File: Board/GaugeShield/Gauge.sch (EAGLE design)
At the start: 29 parts

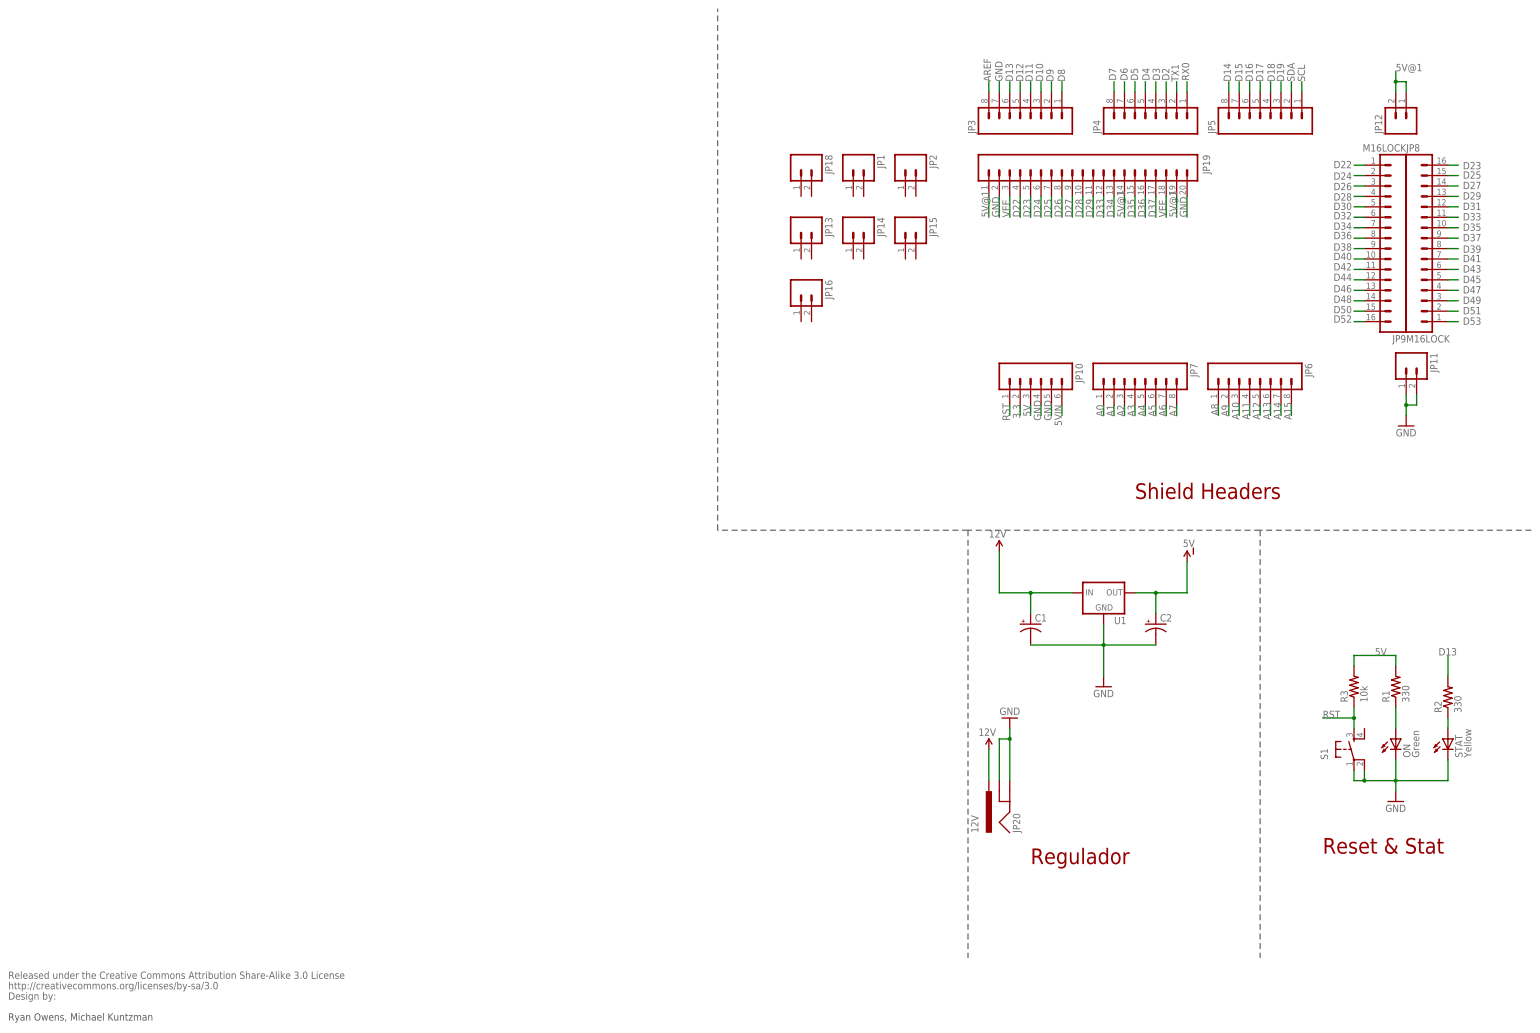
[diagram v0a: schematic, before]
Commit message: empece a diagramar la parte del board y a tracear las rutas
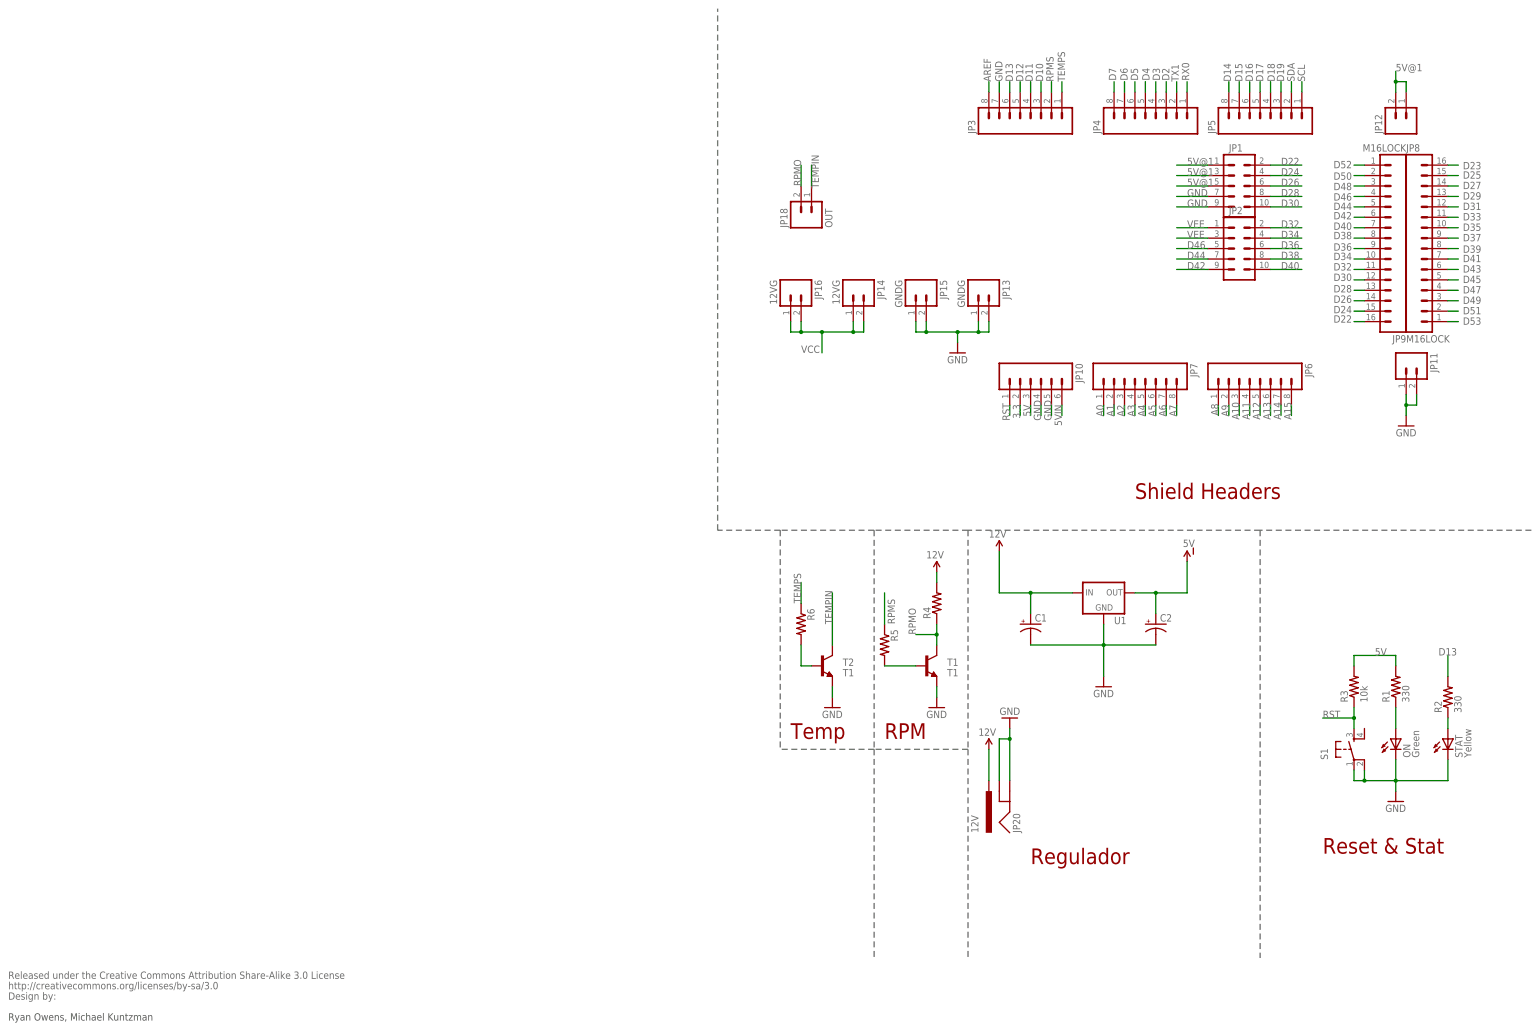
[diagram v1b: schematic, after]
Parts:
- removed JP19: (no value), SparkFun-Connectors:M20
- added R4, R5, R6: (no value), SparkFun-Passives:RESISTORPTH-1/2W
- added T1, T2: T1, SparkFun-DiscreteSemi:TRANSISTOR_NPN_2PTH
- JP1, JP2: device SparkFun-Connectors:M02POLAR -> SparkFun-Connectors:M05X2PTH
- JP13, JP15: value (none) -> GNDG
- JP14, JP16: value (none) -> 12VG
- JP18: value (none) -> OUT
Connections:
- removed net D8: JP3.1
- removed net D9: JP3.2
- new net N$1: R5.2, T1.B
- new net N$2: R6.2, T2.B
- new net RPMO: JP18.2, R4.1, T1.C
- new net RPMS: JP3.2, R5.1
- new net TEMPIN: JP18.1, T2.C
- new net TEMPS: JP3.1, R6.1
- new net VCC: C1.+, JP14.1, JP14.2, JP16.1, JP16.2, JP20.PWR, U1.IN
- net 5V@1: now also JP1.1, JP1.3, JP1.5; no longer JP19.1, JP19.14, JP19.19
- net D22: now also JP1.2, JP9.16; no longer JP19.4, JP9.1
- net D23: no longer JP19.5
- net D24: now also JP1.4, JP9.15; no longer JP19.6, JP9.2
- net D25: no longer JP19.7
- net D26: now also JP1.6, JP9.14; no longer JP19.8, JP9.3
- net D27: no longer JP19.9
- net D28: now also JP1.8, JP9.13; no longer JP19.10, JP9.4
- net D29: no longer JP19.11
- net D30: now also JP1.10, JP9.12; no longer JP9.5
- net D32: now also JP2.2, JP9.11; no longer JP9.6
- net D33: no longer JP19.12
- net D34: now also JP2.4, JP9.10; no longer JP19.13, JP9.7
- net D35: no longer JP19.15
- net D36: now also JP2.6, JP9.9; no longer JP19.16, JP9.8
- net D37: no longer JP19.17
- net D38: now also JP2.8, JP9.8; no longer JP9.9
- net D40: now also JP2.10, JP9.7; no longer JP9.10
- net D42: now also JP2.9, JP9.6; no longer JP9.11
- net D44: now also JP2.7, JP9.5; no longer JP9.12
- net D46: now also JP2.5, JP9.4; no longer JP9.13
- net D48: now also JP9.3; no longer JP9.14
- net D50: now also JP9.2; no longer JP9.15
- net D52: now also JP9.1; no longer JP9.16
- net GND: now also JP1.7, JP1.9, JP13.1, JP13.2, JP15.1, JP15.2, T1.E, T2.E; no longer JP19.2, JP19.20
- net VEE: now also JP2.1, JP2.3; no longer JP19.18, JP19.3
- net VNEG: now also R4.2; no longer C1.+, JP20.PWR, U1.IN
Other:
- note added: "RPM"
- note added: "Temp"
- moved on the sheet: JP13, JP14, JP15, JP16, JP18
